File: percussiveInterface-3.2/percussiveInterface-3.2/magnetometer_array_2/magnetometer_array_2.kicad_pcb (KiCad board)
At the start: 4 copper layers, 167 x 15.9 mm, 52 parts, among them J1 Conn_01x05_Socket, J2 Conn_01x12_Socket, J3 Conn_01x12_Socket, J4 Conn_01x12_Socket, U1 SM225-10E, U10 SM225-10E, U11 SM225-10E, U12 SM225-10E, U13 SM225-10E, U14 SM225-10E, U15 SM225-10E, U16 SM225-10E, U17 SM225-10E, U18 SM225-10E, U19 SM225-10E, U2 SM225-10E, U20 SM225-10E, U21 SM225-10E, U22 SM225-10E, U23 SM225-10E, U24 SM225-10E, U3 SM225-10E, U4 SM225-10E, U5 SM225-10E, U6 SM225-10E, U7 SM225-10E, U8 SM225-10E, U9 SM225-10E

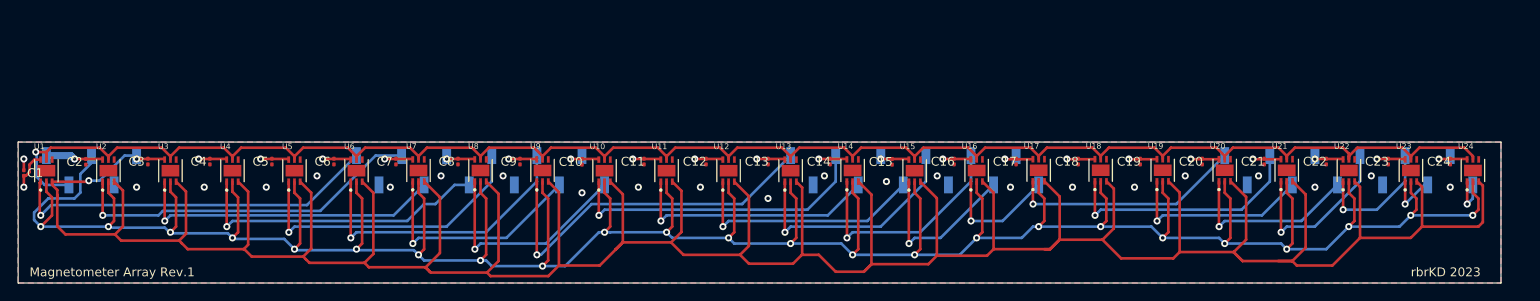
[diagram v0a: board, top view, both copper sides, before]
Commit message: new arrray
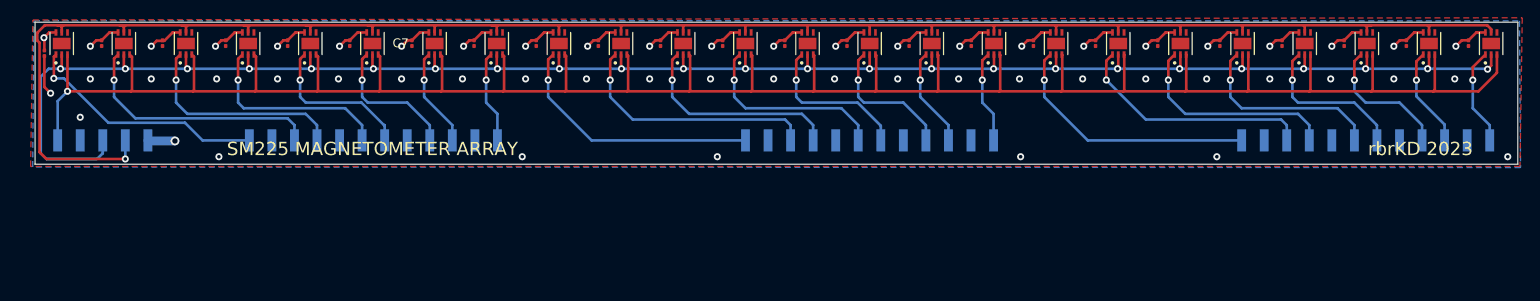
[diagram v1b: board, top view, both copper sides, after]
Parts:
- J1: footprint Connector_PinSocket_2.54mm:PinSocket_1x05_P2.54mm_Vertical_SMD_Pin1Left -> Connector_Harwin:Harwin_M20-89005xx_1x05_P2.54mm_Horizontal
- J2, J3, J4: footprint Connector_PinSocket_2.54mm:PinSocket_1x12_P2.54mm_Vertical_SMD_Pin1Left -> Connector_Harwin:Harwin_M20-89012xx_1x12_P2.54mm_Horizontal
- moved J2 15.0 mm to (78.1, 57.8), turned to 90 degrees
- moved U15 14.5 mm to (141.0, 52.4)
- moved U13 14.5 mm to (127.0, 52.4)
- moved U12 14.4 mm to (120.0, 52.4)
- moved U11 14.4 mm to (113.0, 52.4)
- moved U24 14.4 mm to (204.0, 52.4)
- moved U10 14.4 mm to (106.0, 52.4)
- moved U23 14.4 mm to (197.0, 52.4)
- moved U22 14.4 mm to (190.0, 52.4)
- moved U6 14.4 mm to (78.0, 52.4)
- moved U5 14.4 mm to (71.0, 52.4)
- moved U4 14.4 mm to (64.0, 52.4)
- moved U16 14.4 mm to (148.0, 52.4)
- moved U3 14.4 mm to (57.0, 52.4)
- moved U2 14.4 mm to (50.0, 52.4)
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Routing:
- net MOSI: track 350.9 -> 220.4 mm
- net MISO: track 390.4 -> 267.2 mm
- net SS6: track 32.8 -> 15.6 mm
- net SCLK: track 197.4 -> 214.2 mm
- net SS5: track 33.8 -> 17.5 mm
- net SS7: track 26.2 -> 11.2 mm
- net SS8: track 25.2 -> 10.4 mm
- net SS1: track 42.2 -> 27.7 mm
- net v+: track 81.0 -> 93.9 mm, vias 24 -> 25
- net SS9: track 41.5 -> 29.3 mm
- net SS4: track 34.3 -> 22.3 mm
- net SS2: track 40.2 -> 28.3 mm
- net SS3: track 35.3 -> 24.2 mm
- net SS14: track 25.9 -> 15.7 mm
- net SS13: track 26.9 -> 17.5 mm
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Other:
- board size 167 x 15.9 mm -> 167 x 16 mm
- board text added: "CLCK"
- board text added: "CS1"
- board text added: "CS10"
- board text added: "CS11"
- board text added: "CS12"
- board text added: "CS13"
- board text added: "CS14"
- board text added: "CS15"
- board text added: "CS16"
- board text added: "CS17"
- board text added: "CS18"
- board text added: "CS19"
- board text added: "CS2"
- board text added: "CS20"
- board text added: "CS21"
- board text added: "CS22"
- board text added: "CS23"
- board text added: "CS24"
- board text added: "CS3"
- board text added: "CS4"
- board text added: "CS5"
- board text added: "CS6"
- board text added: "CS7"
- board text added: "CS8"
- board text added: "CS9"
- board text added: "GND"
- board text added: "MISO"
- board text added: "MOSI"
- board text added: "SM225 MAGNETOMETER ARRAY"
- board text added: "V+"
- board text removed: "Magnetometer Array Rev.1"
